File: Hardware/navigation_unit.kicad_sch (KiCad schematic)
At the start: 36 parts, among them SW1 SW_SPDT, SW2 SW_Push_Dual, U4 STM32F405RGTx, Y1 25MHz

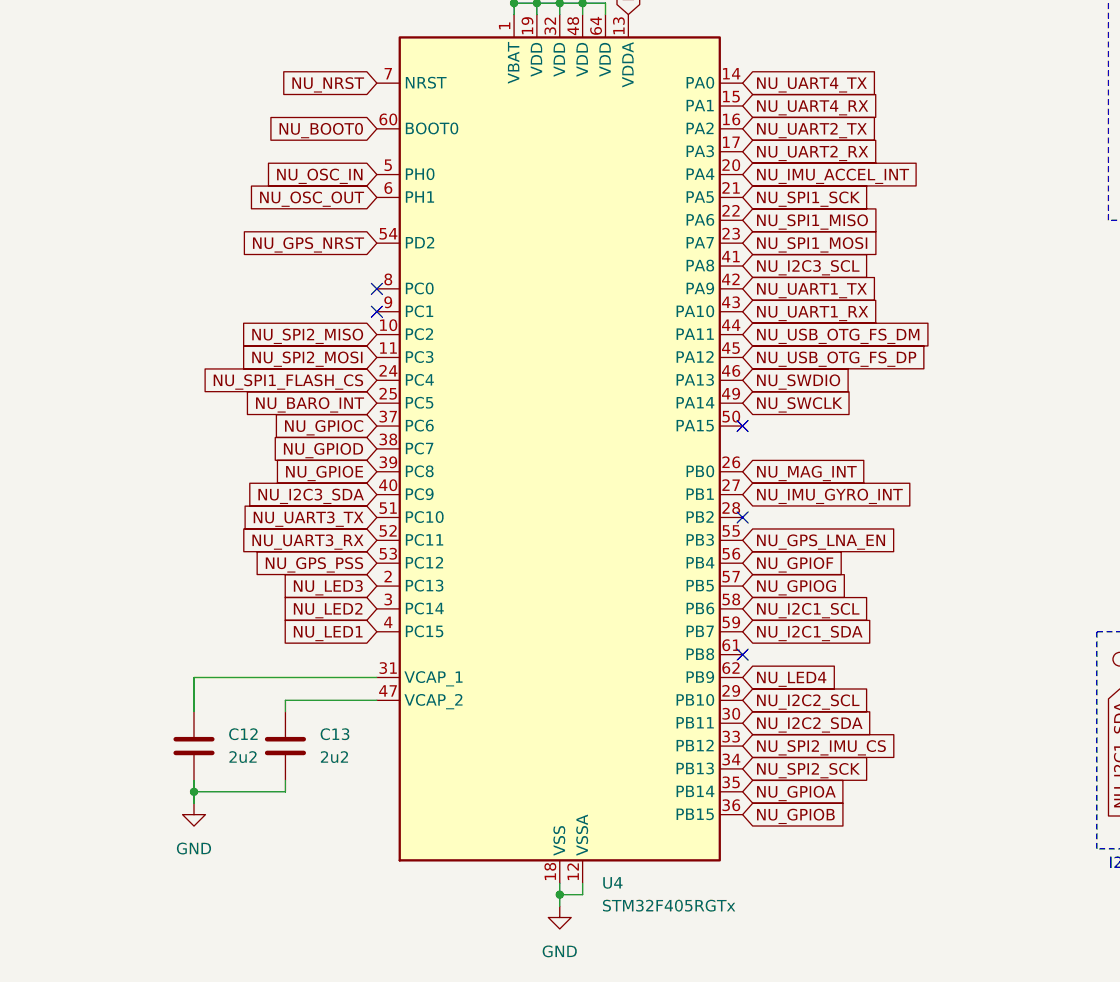
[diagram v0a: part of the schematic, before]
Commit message: pin refatoration, freertos code
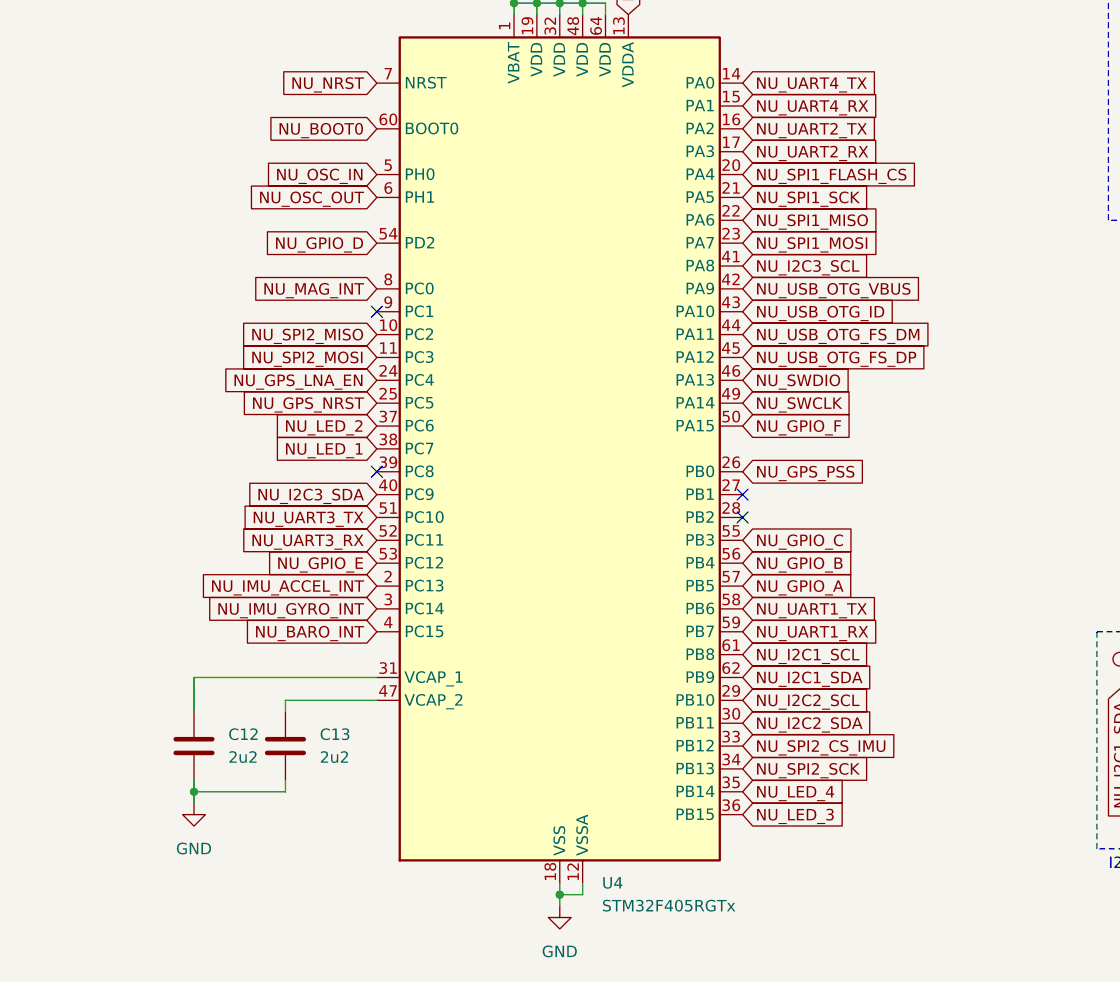
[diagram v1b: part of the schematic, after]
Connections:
- net NU_BARO_INT: now also U4.4 (PC15); no longer U4.25 (PC5)
- net NU_GPS_LNA_EN: now also U4.24 (PC4); no longer U4.55 (PB3)
- net NU_GPS_NRST: now also U4.25 (PC5); no longer U4.54 (PD2)
- net NU_GPS_PSS: now also U4.26 (PB0); no longer U4.53 (PC12)
- net NU_I2C1_SCL: now also U4.61 (PB8); no longer U4.58 (PB6)
- net NU_I2C1_SDA: now also U4.62 (PB9); no longer U4.59 (PB7)
- net NU_IMU_ACCEL_INT: now also U4.2 (PC13); no longer U4.20 (PA4)
- net NU_IMU_GYRO_INT: now also U4.3 (PC14); no longer U4.27 (PB1)
- net NU_LED1: no longer U4.4 (PC15)
- net NU_LED2: no longer U4.3 (PC14)
- net NU_LED3: no longer U4.2 (PC13)
- net NU_LED4: no longer U4.62 (PB9)
- net NU_MAG_INT: now also U4.8 (PC0); no longer U4.26 (PB0)
- net NU_SPI1_FLASH_CS: now also U4.20 (PA4); no longer U4.24 (PC4)
- net NU_UART1_RX: now also U4.59 (PB7); no longer U4.43 (PA10)
- net NU_UART1_TX: now also U4.58 (PB6); no longer U4.42 (PA9)
- net NU_GPIO_F: now reaches U4.50 (PA15)
- net NU_GPIOA renamed NU_LED_4
- net NU_GPIOB renamed NU_LED_3
- net NU_GPIOC renamed NU_LED_2
- net NU_GPIOD renamed NU_LED_1
- net NU_GPIOE: no longer names the net of U4.39 (PC8)
- net NU_GPIOF renamed NU_GPIO_B
- net NU_GPIOG renamed NU_GPIO_A
- net NU_SPI2_IMU_CS renamed NU_SPI2_CS_IMU
- new net NU_GPIO_C: U4.55 (PB3)
- new net NU_GPIO_D: U4.54 (PD2)
- new net NU_GPIO_E: U4.53 (PC12)
- new net NU_USB_OTG_ID: U4.43 (PA10)
- new net NU_USB_OTG_VBUS: U4.42 (PA9)
- no-connect marks 5 -> 4
